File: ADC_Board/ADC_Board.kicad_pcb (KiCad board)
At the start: 2 copper layers, 114 x 66 mm, 51 parts, among them IC1 UCC12040DVE, IC2 ADS131M04QPWRQ1, IC7 ISO7762FDWR, J1 Conn_01x01_Pin, J2 Conn_01x01_Pin, J3 Conn_01x01_Pin, J4 Conn_01x01_Pin, J5 Conn_01x01_Pin, J6 Conn_01x01_Pin, J7 Conn_01x01_Pin, J8 Conn_01x01_Pin, U1 OPA990IDCKR, U2 OPA990IDCKR, U3 INA210AIDCKR, U4 INA210AIDCKR, U5 Nucleo_L432KC

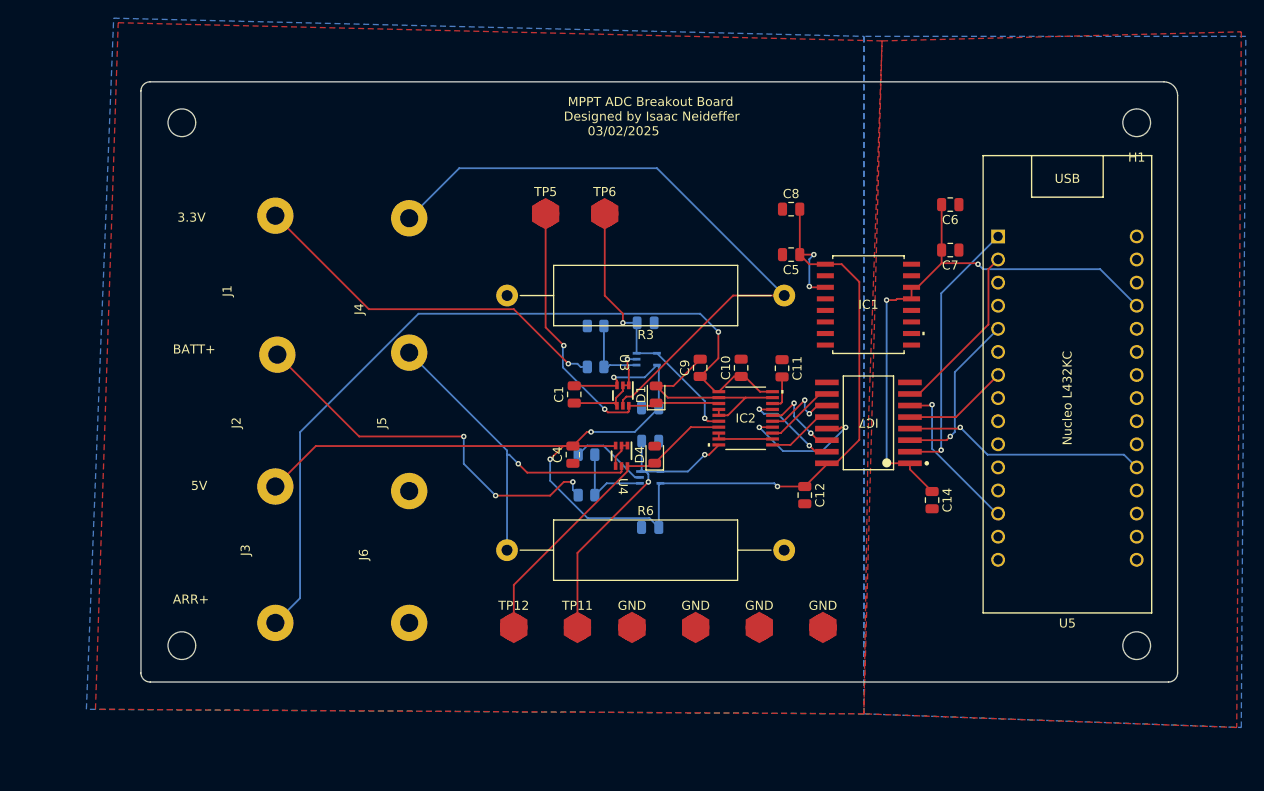
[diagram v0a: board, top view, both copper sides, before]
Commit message: made changes to layout and schematic
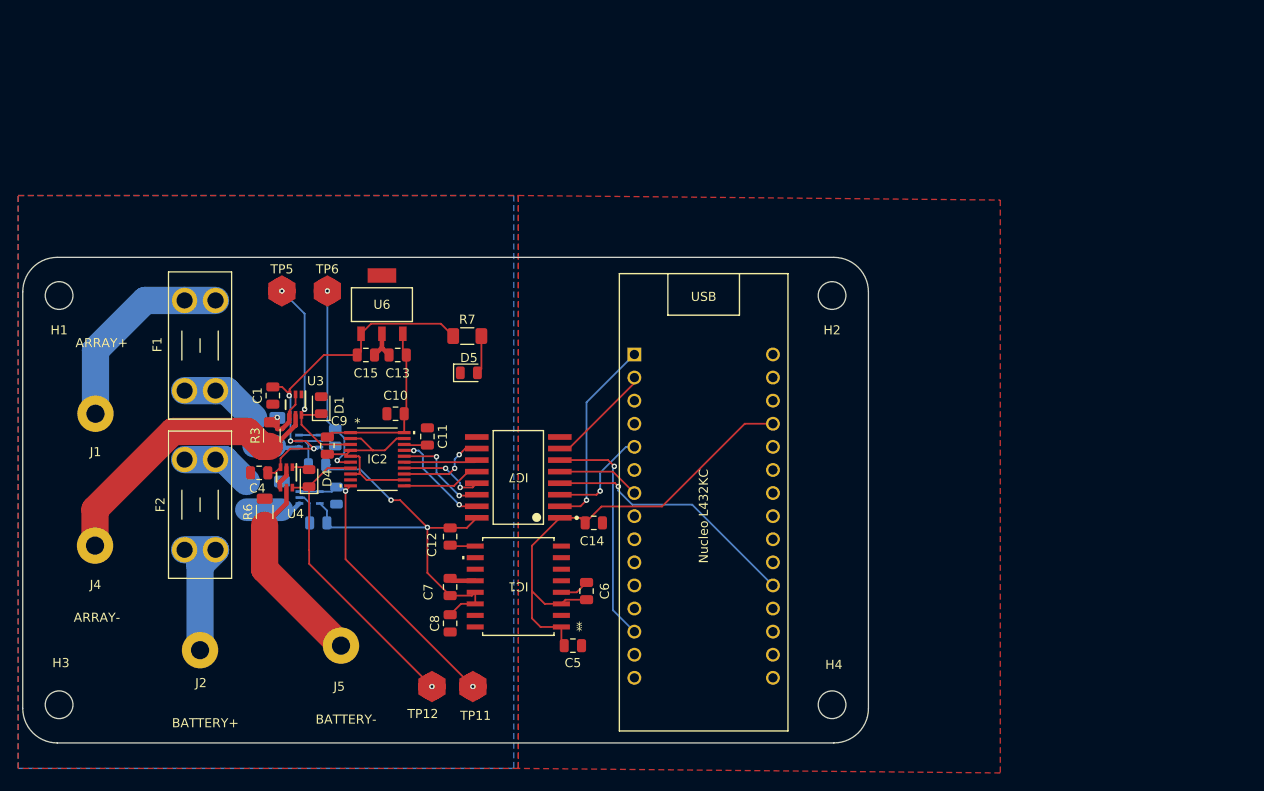
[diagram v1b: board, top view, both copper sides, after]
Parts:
- removed GND (x3): GND_TP, UTSVT_Special:TestPoint_HEX_3mmID
- removed GND: -BATT_TP, UTSVT_Special:TestPoint_HEX_3mmID
- removed J3, J6, J7, J8: Conn_01x01_Pin, UTSVT_Connectors:Banana_Jack_1_Pin_4mm
- added C13: 33u, Capacitor_SMD:C_0805_2012Metric, F.Cu at (187.2, 63.5)
- added C15: 0.47u, Capacitor_SMD:C_0805_2012Metric, F.Cu at (183.7, 63.5)
- added D5: Power_LED, LED_SMD:LED_0805_2012Metric, F.Cu at (195.1, 65.5)
- added F1: Fuse, Fuse:Fuseholder_Blade_Mini_Keystone_3568, F.Cu at (167.2, 57.5)
- added F2: Fuse, Fuse:Fuseholder_Blade_Mini_Keystone_3568, F.Cu at (163.8, 85.0)
- added R7: 3k, Resistor_SMD:R_1206_3216Metric_Pad1.30x1.75mm_HandSolder, F.Cu at (194.9, 61.5)
- added U6: LM3940IMP-3.3, LM3940:MP04A, F.Cu at (185.5, 58.0)
- C5: value 10u -> 0.1u
- C6: value 0.1u -> 10u
- R1, R2, R4, R5: footprint Resistor_SMD:R_0805_2012Metric -> Resistor_SMD:R_1206_3216Metric_Pad1.30x1.75mm_HandSolder
- R3, R6: footprint Resistor_THT:R_Axial_Power_L20.0mm_W6.4mm_P30.48mm -> Resistor_SMD:R_1206_3216Metric
- moved H1 120.0 mm to (150.0, 57.0)
- moved H4 71.8 mm to (235.0, 102.0)
- moved C7 66.3 mm to (193.0, 89.0), turned to -90 degrees
- moved H3 65.4 mm to (150.0, 102.0)
- moved C8 59.0 mm to (193.0, 93.0), turned to 90 degrees
- moved R3 58.4 mm to (173.4, 72.4), turned to 90 degrees
- moved C6 58.4 mm to (208.0, 89.5), turned to 90 degrees
- moved H2 51.0 mm to (235.0, 57.0)
- moved J4 49.9 mm to (153.9, 84.5), turned to 0 degrees
- moved IC1 49.4 mm to (200.5, 89.0), turned to 180 degrees
- moved C5 49.2 mm to (206.5, 95.5)
- moved U5 42.1 mm to (220.9, 81.3)
- moved C9 41.9 mm to (179.5, 73.5), turned to -90 degrees
- moved IC2 40.7 mm to (185.0, 75.0)
- moved C11 39.7 mm to (190.5, 72.5)
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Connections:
- C5 pad 1: +5V -> GND_I
- C5 pad 2: GND -> +5V_I
- C6 pad 1: GND_I -> +5V_I
- C6 pad 2: +5V_I -> GND_I
- C7 pad 1: GND_I -> GND
- C7 pad 2: +5V_I -> +5V
- IC1 pad 1: +5V -> +5V_I
- IC1 pad 10: GND_I -> GND
- IC1 pad 11: GND_I -> GND
- IC1 pad 12: GND_I -> GND
- IC1 pad 13: +5V_I -> +5V
- IC1 pad 14: +5V_I -> +5V
- IC1 pad 15: GND_I -> GND
- IC1 pad 16: GND_I -> GND
- IC1 pad 2: GND -> GND_I
- IC1 pad 3: +5V -> +5V_I
- IC1 pad 4: GND -> GND_I
- IC1 pad 6: GND -> GND_I
- IC1 pad 7: GND -> GND_I
- IC1 pad 8: GND -> GND_I
- IC1 pad 9: GND_I -> GND
- R1 pad 2: /ARR+ -> /ARR+_IN
- R4 pad 2: /BATTERY+ -> /BATT+_IN
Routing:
- net +3.3V: track 90.1 -> 19.8 mm, vias 1 -> 0
- net +5V: track 152.2 -> 94.6 mm, vias 6 -> 5
- net /ARR-: track 72.5 -> 32.2 mm
- net /BATTERY+: track 43.0 -> 15.1 mm, vias 3 -> 0
- net /ARR+: track 41.2 -> 22.5 mm, vias 1 -> 0
- net /BATTERY-: track 40.3 -> 21.8 mm, vias 1 -> 0
- net /ARRAY_CURRENT+: track 37.8 -> 24.4 mm
- net /ARR+_IN: track 0.00 -> 8.84 mm
- net /ADC_DRIVER_CLK_I: track 29.6 -> 21.4 mm
- net /MISO_I: track 17.5 -> 25.5 mm
- net /BATT+_IN: track 0.00 -> 7.80 mm
- net +5V_I: track 63.0 -> 55.4 mm, vias 3 -> 0
- net /DRDY_I: track 19.4 -> 11.8 mm
- net /MOSI_I: track 18.6 -> 11.6 mm
- net /SPI_CLOCK: track 15.2 -> 9.35 mm
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- removed copper zone on B.Cu, net GND_I
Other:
- board size 114 x 66 mm -> 93 x 53.4 mm
- board text added: "ARRAY+"
- board text added: "ARRAY-"
- board text added: "BATTERY+"
- board text added: "BATTERY-"
- board text removed: "3.3V"
- board text removed: "5V"
- board text removed: "ARR+"
- board text removed: "BATT+"
- board text removed: "MPPT ADC Breakout Board Designed by Isaac Neideffer 03/02/2025"
